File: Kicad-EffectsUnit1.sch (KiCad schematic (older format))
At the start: 104 parts, among them J101 In7, J102 Doepfer connector, J104 In6, J105 In3, J106 Out10, J107 Out11, J108 Out9, J109 Out6, SW101 Dist 6, SW102 Crush A6, SW104 Rotary_Encoder_Switch, SW105 Dist 10, U101 TL072, U102 TL072

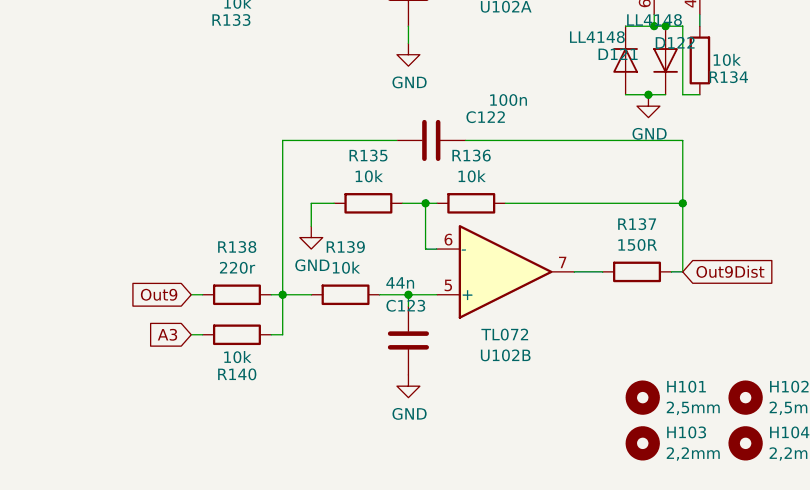
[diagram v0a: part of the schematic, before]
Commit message: filters 2
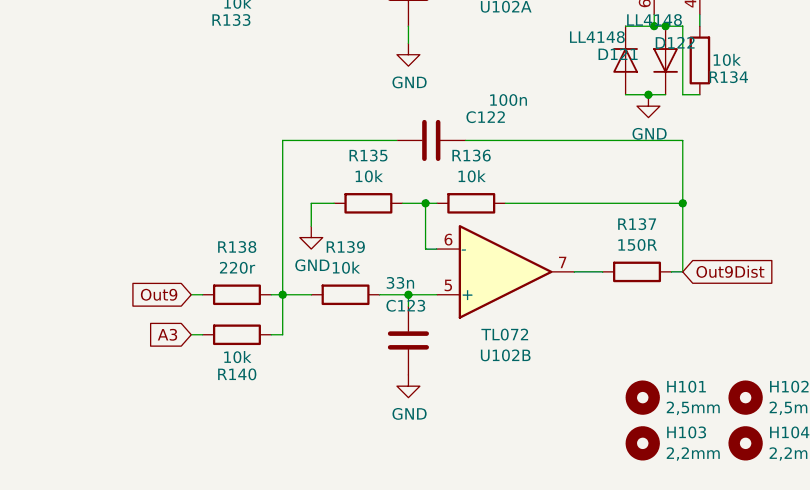
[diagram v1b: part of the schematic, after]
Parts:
- C123: value 44n -> 33n
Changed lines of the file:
@@
 P 5050 7175
 F 0 "C123" H 4950 7325 50  0000 L CNN
-F 1 "44n" H 4950 7425 50  0000 L CNN
+F 1 "33n" H 4950 7425 50  0000 L CNN
 F 2 "Capacitor_SMD:C_0805_2012Metric_Pad1.15x1.40mm_HandSolder" H 5088 7025 50  0001 C CNN
 F 3 "~" H 5050 7175 50  0001 C CNN
